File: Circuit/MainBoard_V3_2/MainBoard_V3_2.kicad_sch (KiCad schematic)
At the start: 143 parts, among them J1 Conn_01x02, J10 Conn_01x03, J11 Conn_01x03, J12 Conn_01x04, J13 Conn_01x04, J14 Conn_01x04, J15 Conn_01x04, J2 Conn_01x02, J3 Conn_01x02, J4 Conn_01x04, J5 Conn_01x02, J6 Conn_01x02, J7 Conn_01x02, J8 Conn_01x07, J9 Raspberry_Pi_2_3, Q1 Q_PMOS_GDS, Q10 BSS138, Q2 Q_PMOS_GDS, Q3 BSS138, Q4 IRLML6402, Q5 BSS138, Q6 BSS138, Q7 BSS138, Q8 BSS138, Q9 BSS138, SW1 SW_Push, SW2 SW_Push, SW3 SW_Push, SW4 SW_Slide_DPDT, SW5 SW_Slide_DPDT, U1 STM32F446RETx, U2 LM1117MP-3.3, U3 MPU-6050, U4 INA180A2, U5 INA180A2, Y1 CSTNE16M0V530000R0

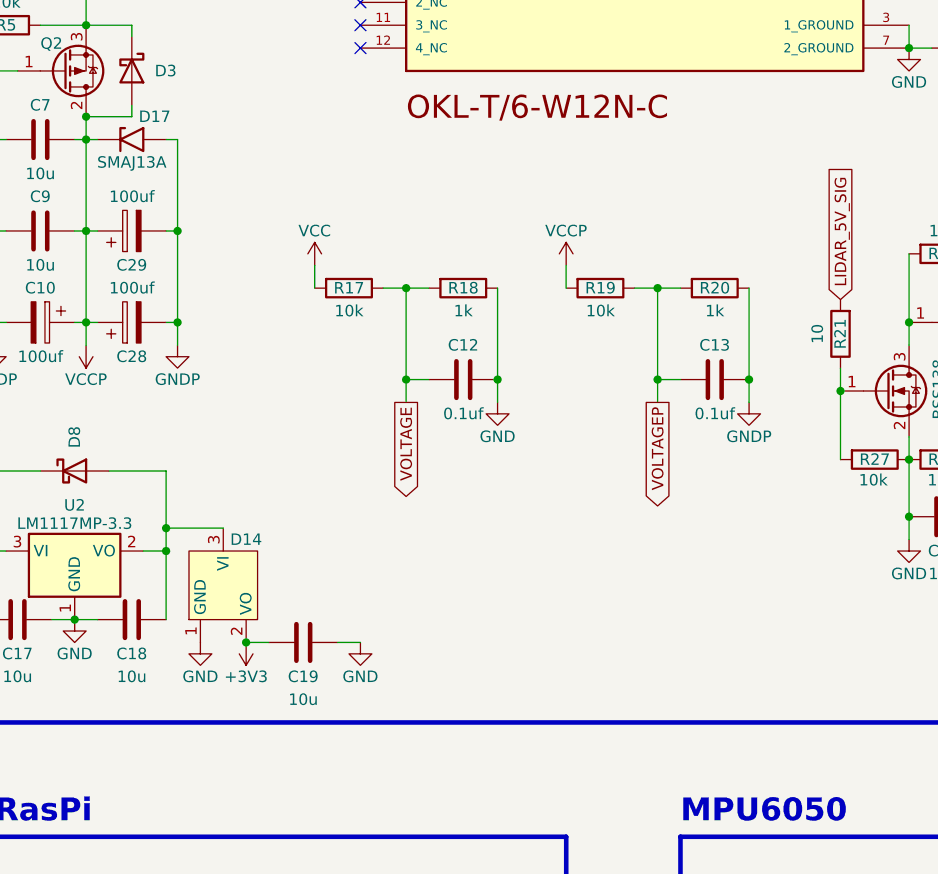
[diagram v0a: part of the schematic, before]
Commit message: 修正多分最終
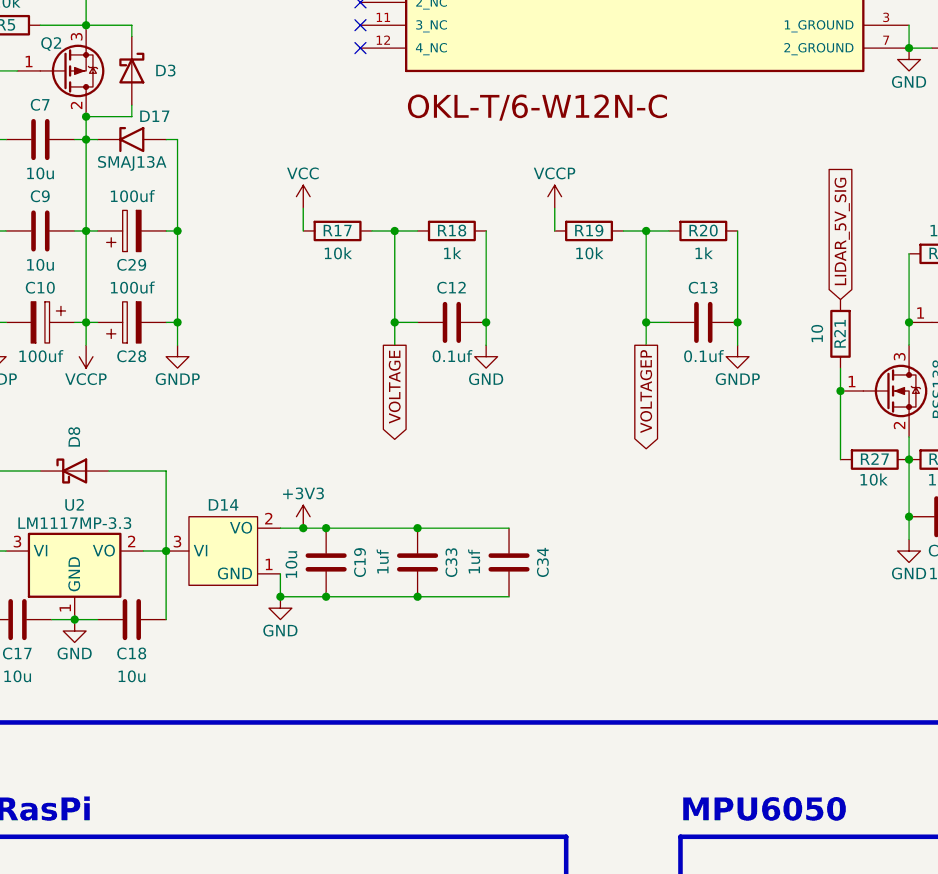
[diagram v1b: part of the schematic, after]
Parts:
- added C33, C34: 1uf, Capacitor_SMD:C_0603_1608Metric, symbol Device:C
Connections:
- net +3V3: now also C33.2, C34.2
- net GND: now also C33.1, C34.1
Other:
- moved on the sheet: C12, C13, C19, D14, R17, R18, R19, R20
